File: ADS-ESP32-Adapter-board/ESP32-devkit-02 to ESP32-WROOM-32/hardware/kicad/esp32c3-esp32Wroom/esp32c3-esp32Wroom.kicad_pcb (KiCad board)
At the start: 2 copper layers, 44.5 x 42.5 mm, 8 parts, among them J1 Conn_01x15_esp32_devkit_V1_el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, J2 Conn_01x15_esp32_devkit_V1_el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, J3 Conn_01x15_esp32_c3_devkit_02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, J4 Conn_01x15_esp32_c3_devkit_02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, J5 Conn_01x06

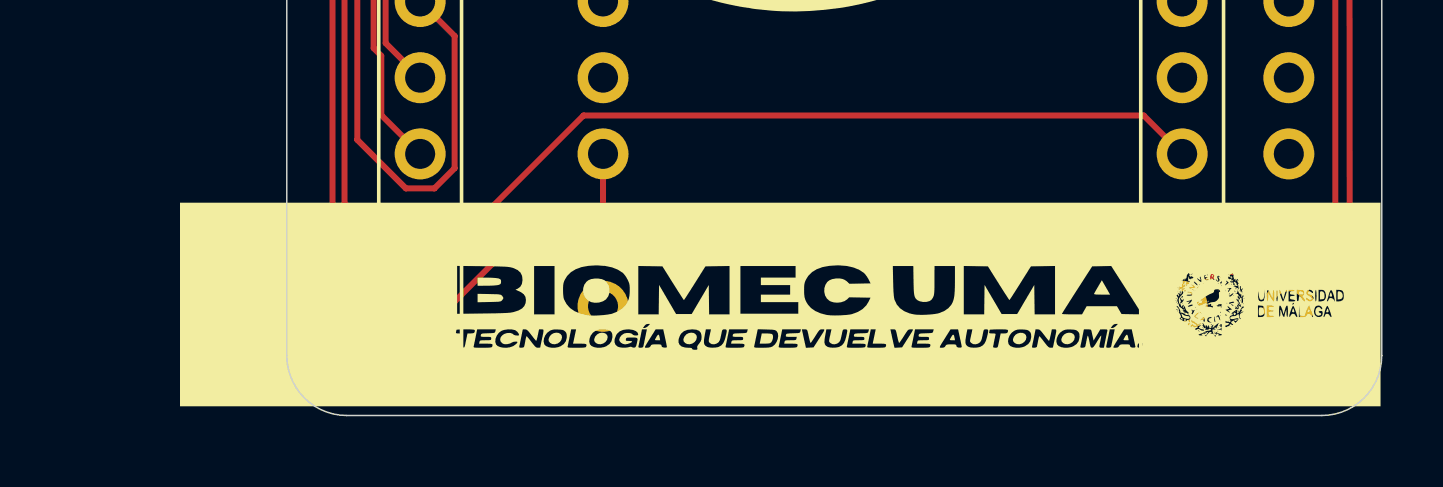
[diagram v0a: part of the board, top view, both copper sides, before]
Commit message: Refactor code structure for improved readability and maintainability
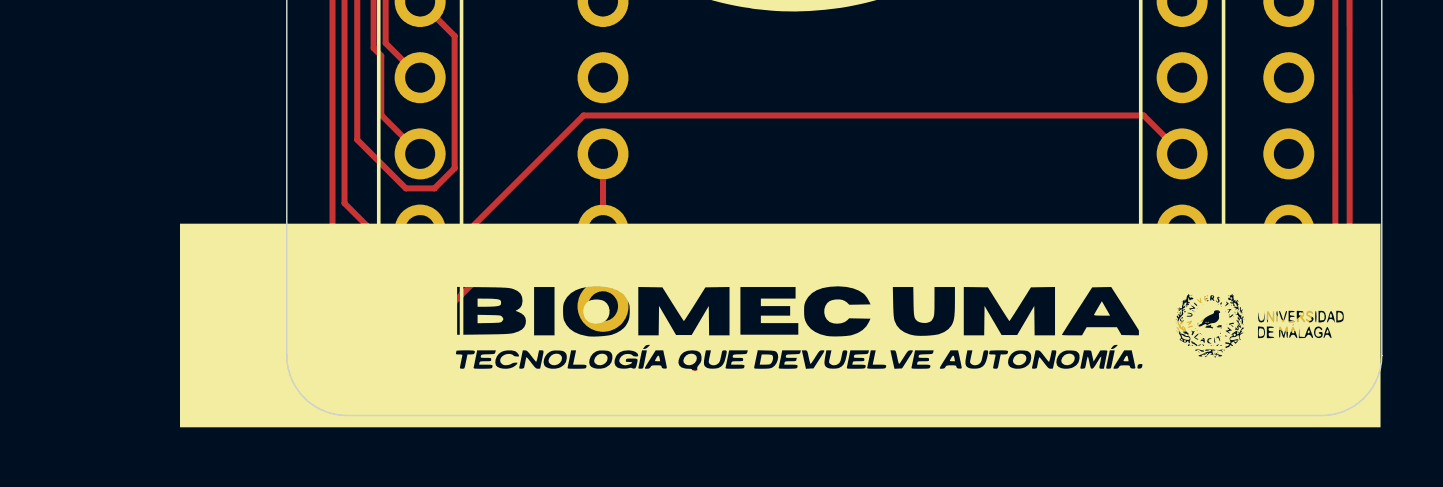
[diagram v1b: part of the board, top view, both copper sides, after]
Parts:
- moved G*** 0.70 mm to (132.1, 94.4)
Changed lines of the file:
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@@
 		(capping no)
 		(filling no)
-		(zone_defaults)
 		(grid_origin 115.6 97.403444)
 		(pcbplotparams
@@
 	(footprint "kicad:biomecumabanner"
 		(layer "F.Cu")
-		(at 132.05 93.703444)
+		(at 132.05 94.403444)
 		(property "Reference" "G***"
 			(at 0 0 0)
